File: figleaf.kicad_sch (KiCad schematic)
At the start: 40 parts, among them U1 Nice_Nano_V2_GRAZ

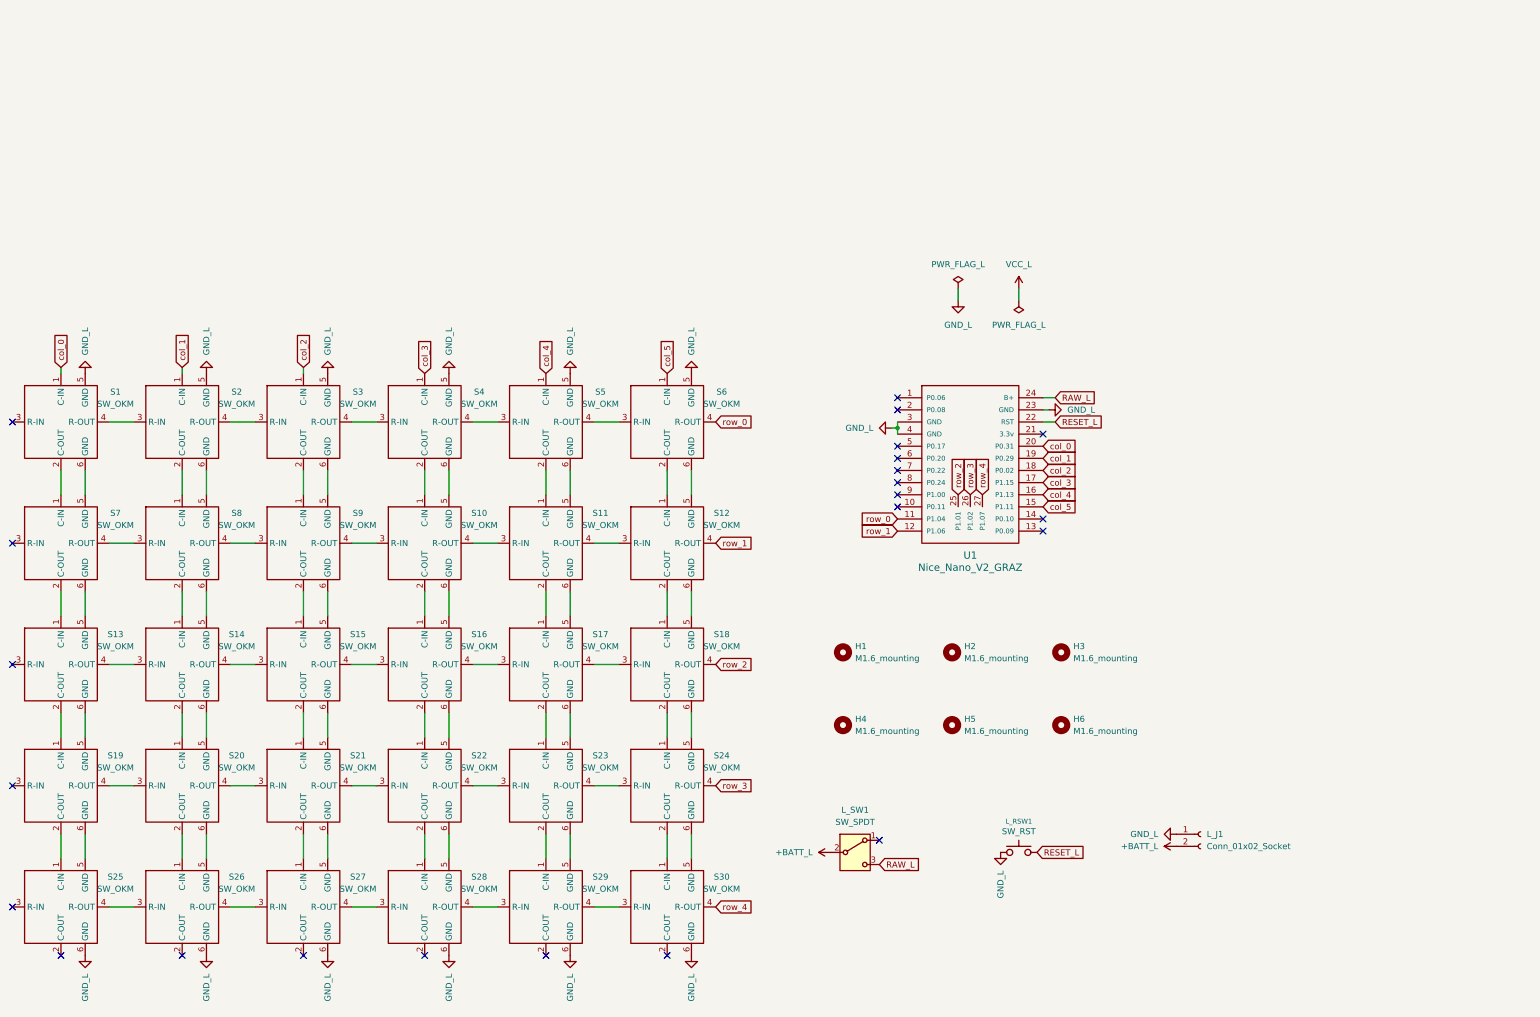
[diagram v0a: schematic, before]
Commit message: start with seeed mcu
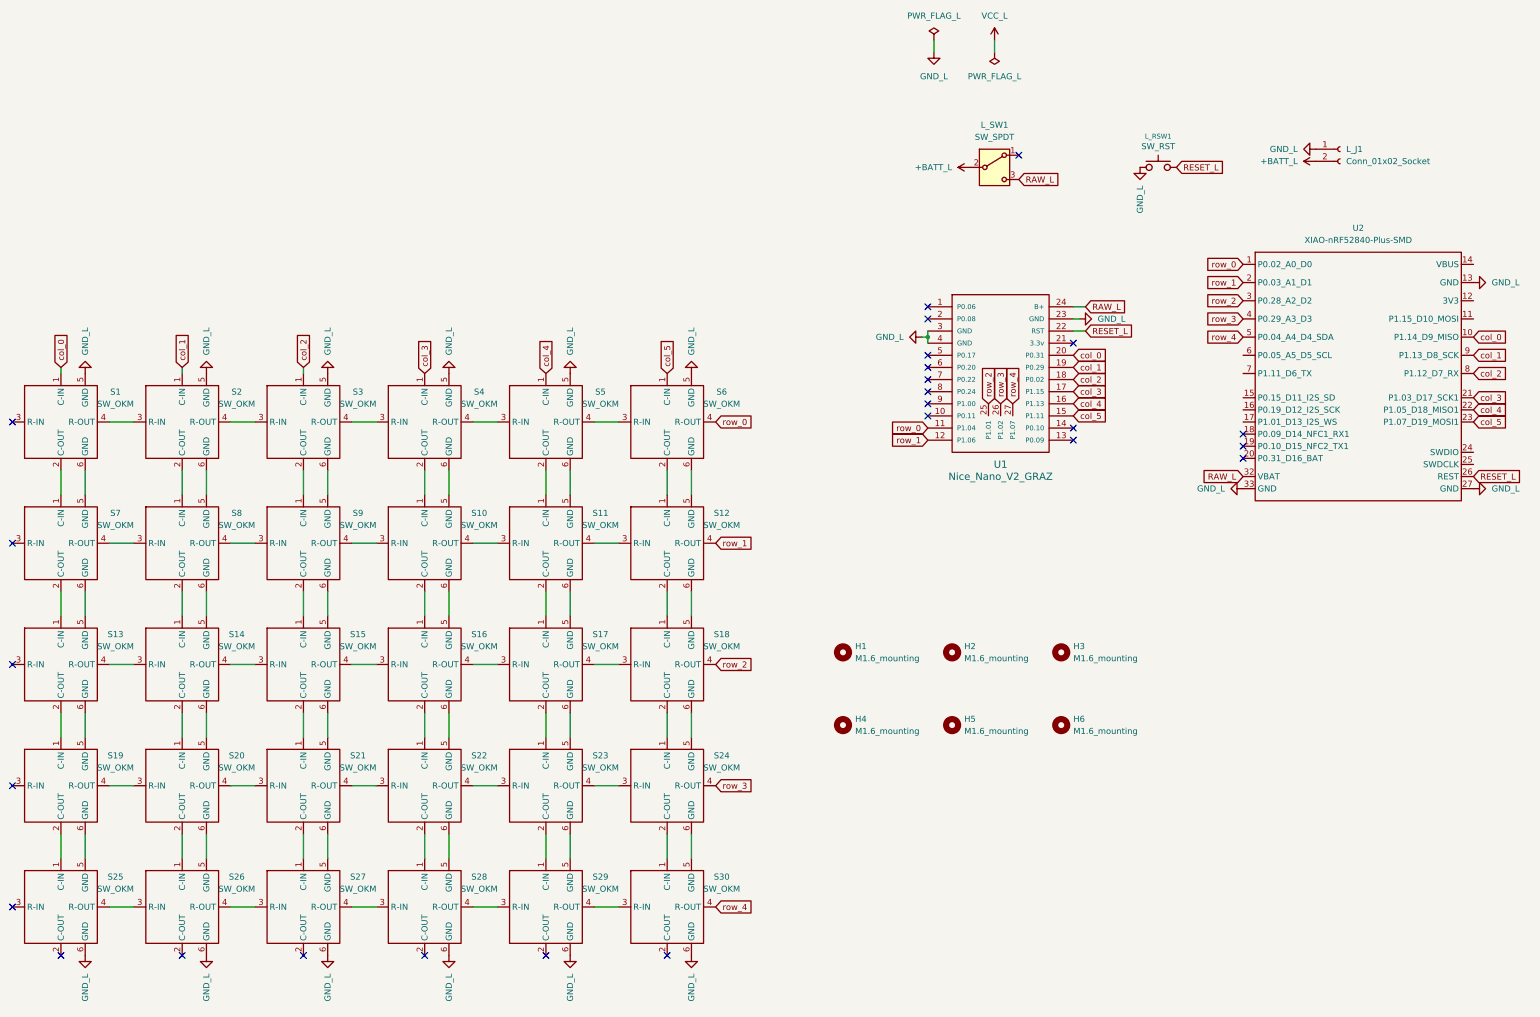
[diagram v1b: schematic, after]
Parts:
- added U2: XIAO-nRF52840-Plus-SMD, Graz_Footprints:XIAO-nRF52840-Plus-SMD, symbol 0_graz_symbols:XIAO-nRF52840_Plus_SMD
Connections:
- net GND_L: now also U2.13 (GND), U2.27 (GND), U2.33 (GND)
- net RAW_L: now also U2.32 (VBAT)
- net RESET_L: now also U2.26 (REST)
- net col_0: now also U2.10 (P1.14_D9_MISO)
- net col_1: now also U2.9 (P1.13_D8_SCK)
- net col_2: now also U2.8 (P1.12_D7_RX)
- net col_3: now also U2.21 (P1.03_D17_SCK1)
- net col_4: now also U2.22 (P1.05_D18_MISO1)
- net col_5: now also U2.23 (P1.07_D19_MOSI1)
- net row_0: now also U2.1 (P0.02_A0_D0)
- net row_1: now also U2.2 (P0.03_A1_D1)
- net row_2: now also U2.3 (P0.28_A2_D2)
- net row_3: now also U2.4 (P0.29_A3_D3)
- net row_4: now also U2.5 (P0.04_A4_D4_SDA)
- no-connect marks 23 -> 26
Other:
- moved on the sheet: L_J1, L_RSW1, L_SW1, U1
